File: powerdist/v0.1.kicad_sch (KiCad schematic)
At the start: 38 parts, among them J1 Conn_01x02_Socket, J2 Conn_01x02_Socket, J3 Conn_01x02_Socket, J4 Conn_01x02_Socket, Q3 SI4178DY, Q4 SI4178DY, Q5 SI4178DY

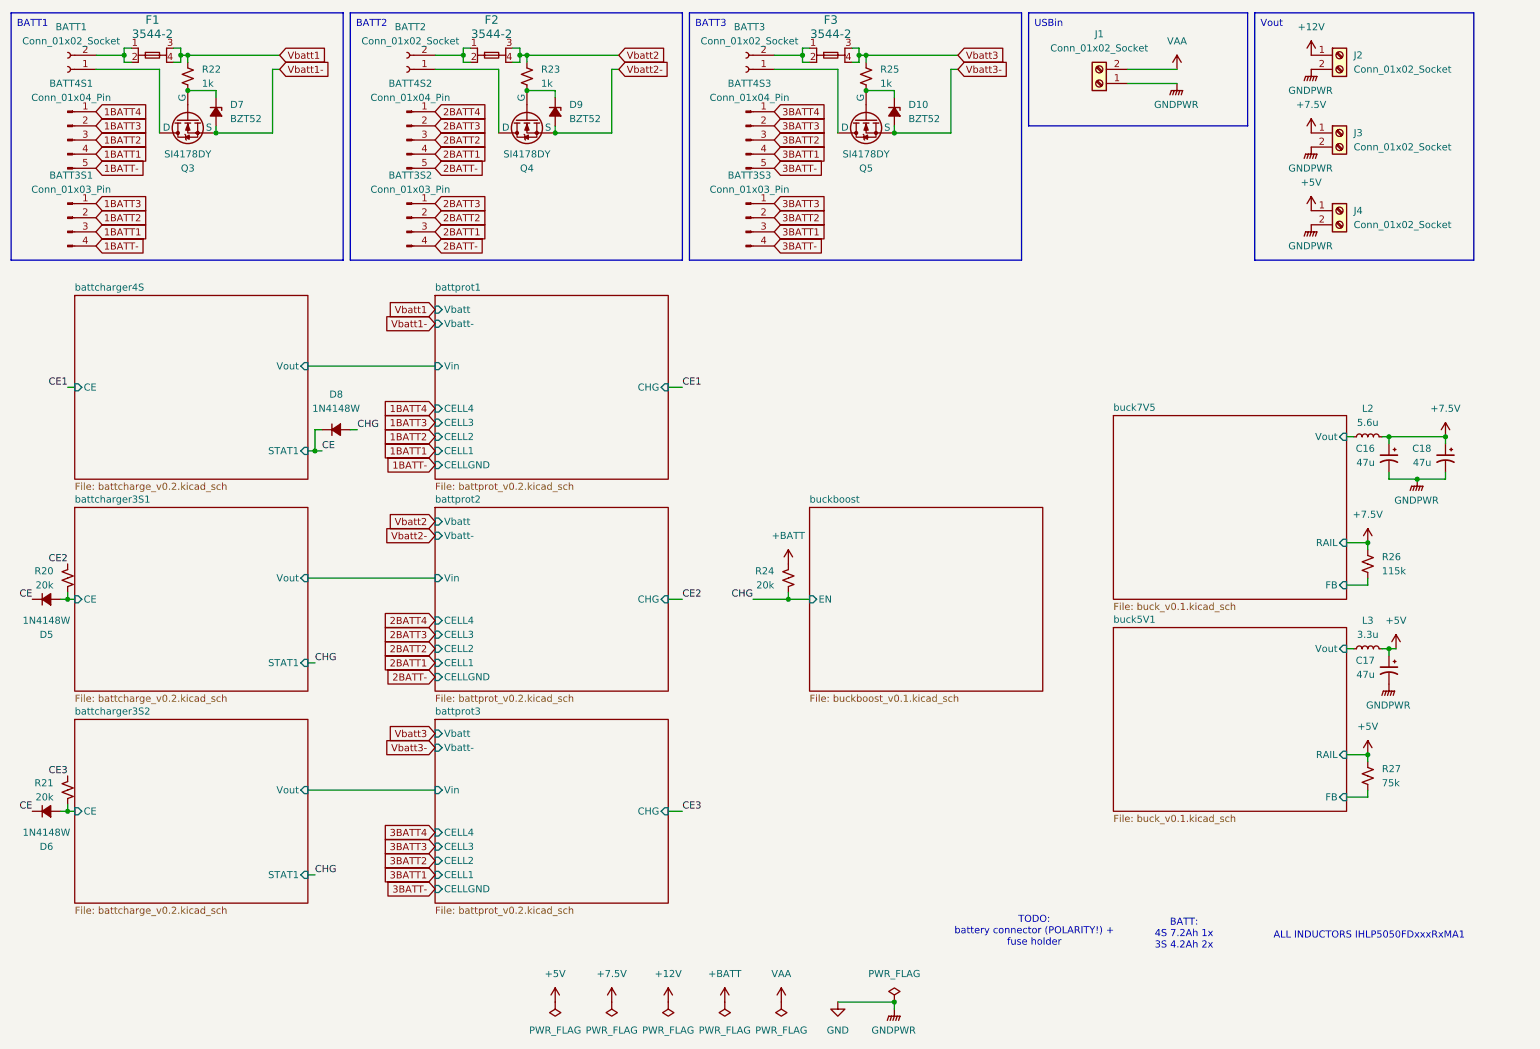
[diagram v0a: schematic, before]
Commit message: lab 23/10
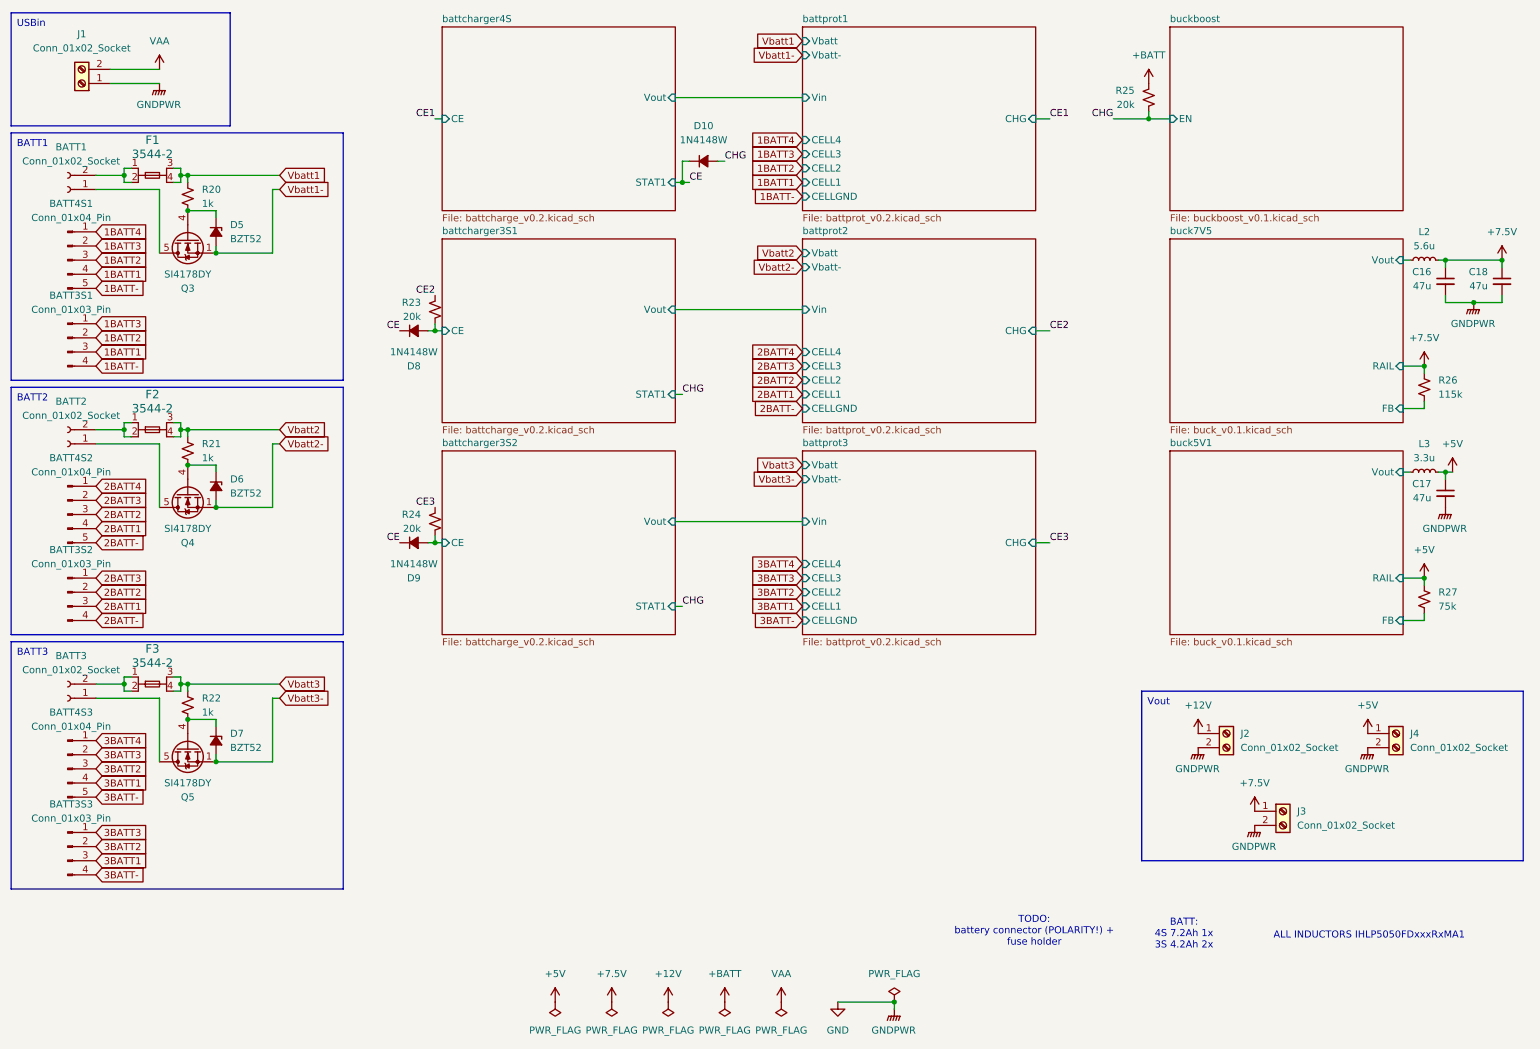
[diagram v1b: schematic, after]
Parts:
- C16, C17, C18: footprint (none) -> Capacitor_SMD:C_1206_3216Metric; symbol Device:C_Polarized_Small_US -> Device:C_Small
- Q3, Q4, Q5: footprint (none) -> Package_SO:PowerPAK_SO-8_Single; symbol Simulation_SPICE:NMOS -> Transistor_FET:Si7336ADP
- renumbered D8 to D10, D7 to D5, D9 to D6, D10 to D7, D5 to D8, D6 to D9, R22 to R20, R23 to R21, R25 to R22, R20 to R23, R21 to R24, R24 to R25
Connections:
- net Vbatt1-: now also Q3.1 (S), Q3.2 (S)
- net Vbatt2-: now also Q4.1 (S), Q4.2 (S)
- net Vbatt3-: now also Q5.1 (S), Q5.2 (S)
- net at BATT1.1 (Pin_1): now also Q3.5 (D); no longer Q3.1 (D)
- net at D6.1 (K), R21.2: now also Q4.4 (G); no longer Q4.2 (G)
- net at BATT3.1 (Pin_1): now also Q5.5 (D); no longer Q5.1 (D)
- net at D7.1 (K), R22.2: now also Q5.4 (G); no longer Q5.2 (G)
- net at BATT2.1 (Pin_1): now also Q4.5 (D); no longer Q4.1 (D)
- net at D5.1 (K), R20.2: now also Q3.4 (G); no longer Q3.2 (G)
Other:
- moved on the sheet: BATT1, BATT2, BATT3, BATT3S1, BATT3S2, BATT3S3, BATT4S1, BATT4S2, BATT4S3, D10, D5, D6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
